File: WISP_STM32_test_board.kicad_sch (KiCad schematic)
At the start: 30 parts, among them J1 Conn_02x05_Odd_Even, J2 Conn_02x01, J3 Conn_02x01, J5 Conn_01x02_Pin, J6 Conn_01x09_Pin, U1 MAX3072E, U2 MAX3072E, U3 AMS1117-3.3, U4 STM32F446RETx

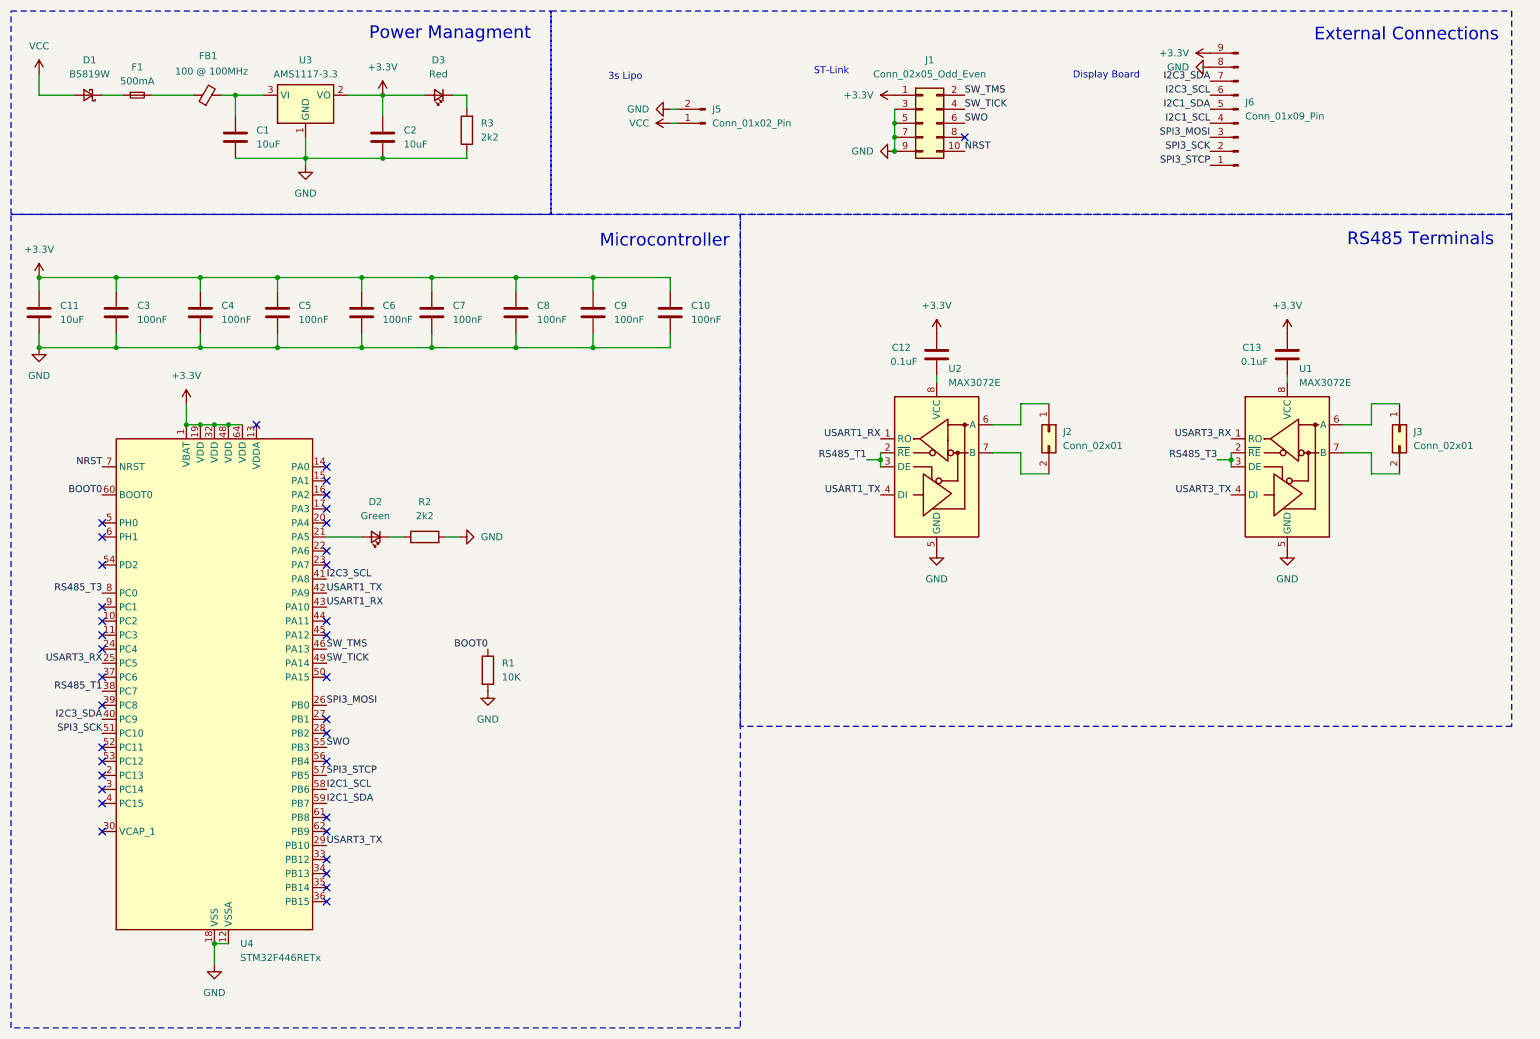
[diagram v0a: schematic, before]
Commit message: Full 15 rough draft
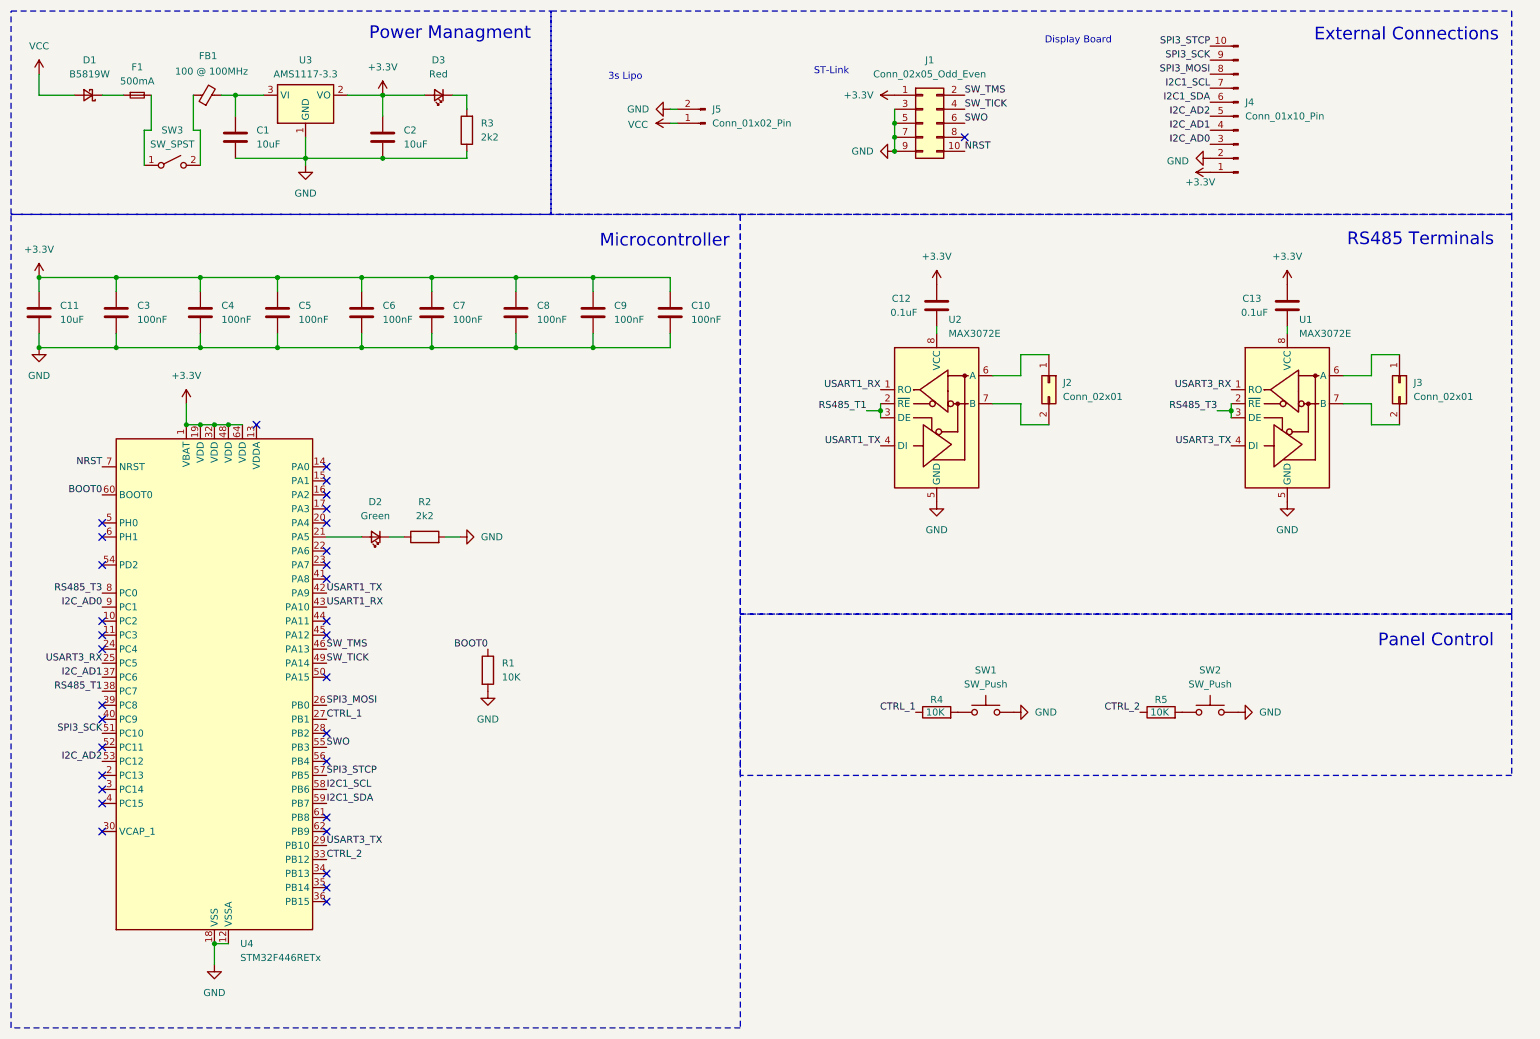
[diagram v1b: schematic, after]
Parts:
- removed J6: Conn_01x09_Pin, Connector_PinSocket_2.54mm:PinSocket_1x09_P2.54mm_Vertical, symbol Connector:Conn_01x09_Pin
- added J4: Conn_01x10_Pin, symbol Connector:Conn_01x10_Pin
- added R4, R5: 10K, Resistor_SMD:R_0805_2012Metric_Pad1.20x1.40mm_HandSolder, symbol Device:R
- added SW1, SW2: SW_Push, Button_Switch_THT:SW_PUSH_6mm, symbol Switch:SW_Push
- added SW3: SW_SPST, symbol Switch:SW_SPST
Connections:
- net +3.3V: now also J4.1 (Pin_1)
- net GND: now also J4.2 (Pin_2), SW1.2, SW2.2
- net I2C1_SCL: now also J4.7 (Pin_7)
- net I2C1_SDA: now also J4.6 (Pin_6)
- net SPI3_MOSI: now also J4.8 (Pin_8)
- net SPI3_SCK: now also J4.9 (Pin_9)
- net SPI3_STCP: now also J4.10 (Pin_10)
- net at F1.2: now also SW3.1 (A); no longer FB1.1
- net CTRL_1: now reaches U4.27 (PB1)
- net CTRL_1: now also R4.1
- net CTRL_2: now reaches U4.33 (PB12)
- net CTRL_2: now also R5.1
- net I2C_AD1: now reaches U4.37 (PC6)
- net I2C_AD1: now also J4.4 (Pin_4)
- net I2C_AD2: now reaches U4.53 (PC12)
- net I2C_AD2: now also J4.5 (Pin_5)
- net I2C_AD0: now reaches U4.9 (PC1)
- net I2C_AD0: now also J4.3 (Pin_3)
- net I2C3_SCL: no longer names the net of U4.41 (PA8)
- net I2C3_SDA: no longer names the net of U4.40 (PC9)
- new net: R5.2, SW2.1
- new net: R4.2, SW1.1
- new net: FB1.1, SW3.2 (B)
- no-connect marks 36 -> 33
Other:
- note added: "Panel Control"
- company: (none) -> Wisconsin Space Program
- title: (none) -> P&ID display control board
- moved on the sheet: C12, C13, J2, J3, U1, U2

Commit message: V1 routing
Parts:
- J4: footprint (none) -> Connector_JST:JST_XH_B10B-XH-A_1x10_P2.50mm_Vertical
- SW3: footprint (none) -> Button_Switch_SMD:SW_DIP_SPSTx01_Slide_6.7x4.1mm_W6.73mm_P2.54mm_LowProfile_JPin
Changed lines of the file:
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@@
 			)
 		)
-		(property "Footprint" ""
+		(property "Footprint" "Button_Switch_SMD:SW_DIP_SPSTx01_Slide_6.7x4.1mm_W6.73mm_P2.54mm_LowProfile_JPin"
 			(at 41.91 40.64 0)
 			(effects
@@
 			)
 		)
-		(property "Footprint" ""
+		(property "Footprint" "Connector_JST:JST_XH_B10B-XH-A_1x10_P2.50mm_Vertical"
 			(at 234.95 31.75 0)
 			(effects
